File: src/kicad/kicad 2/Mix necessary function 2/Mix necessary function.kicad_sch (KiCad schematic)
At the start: 26 parts, among them SW1 02-JST, SW2 02-JST

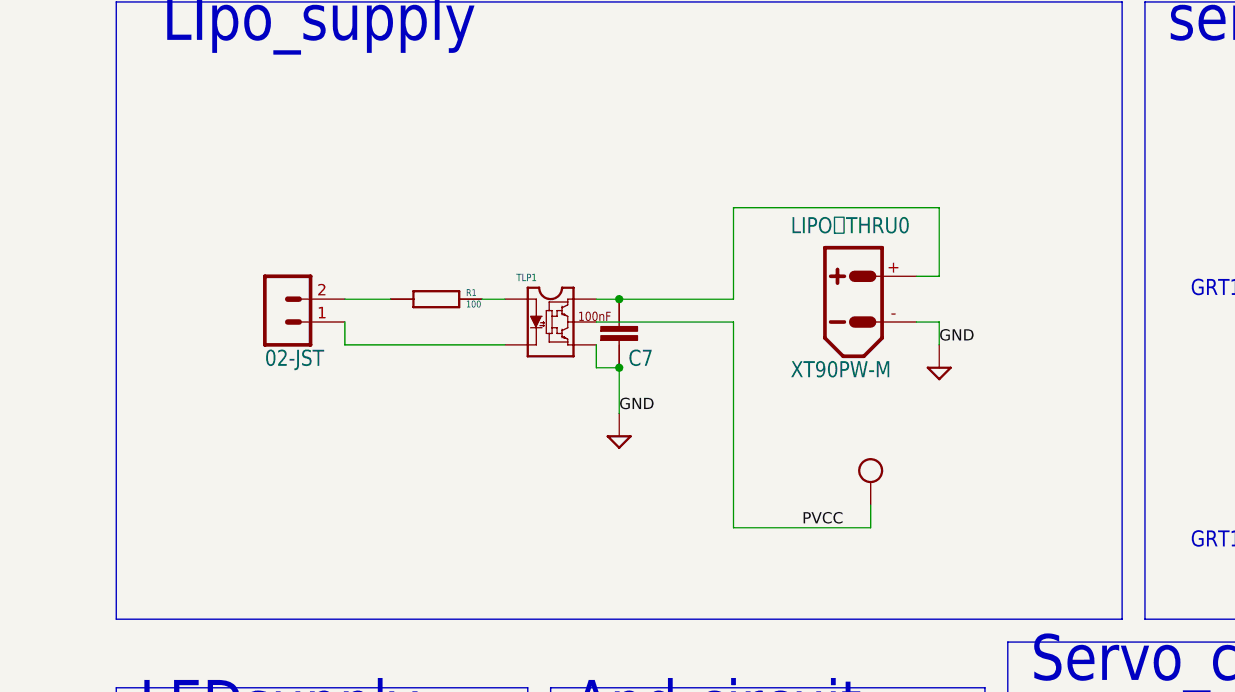
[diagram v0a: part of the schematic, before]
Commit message: fix
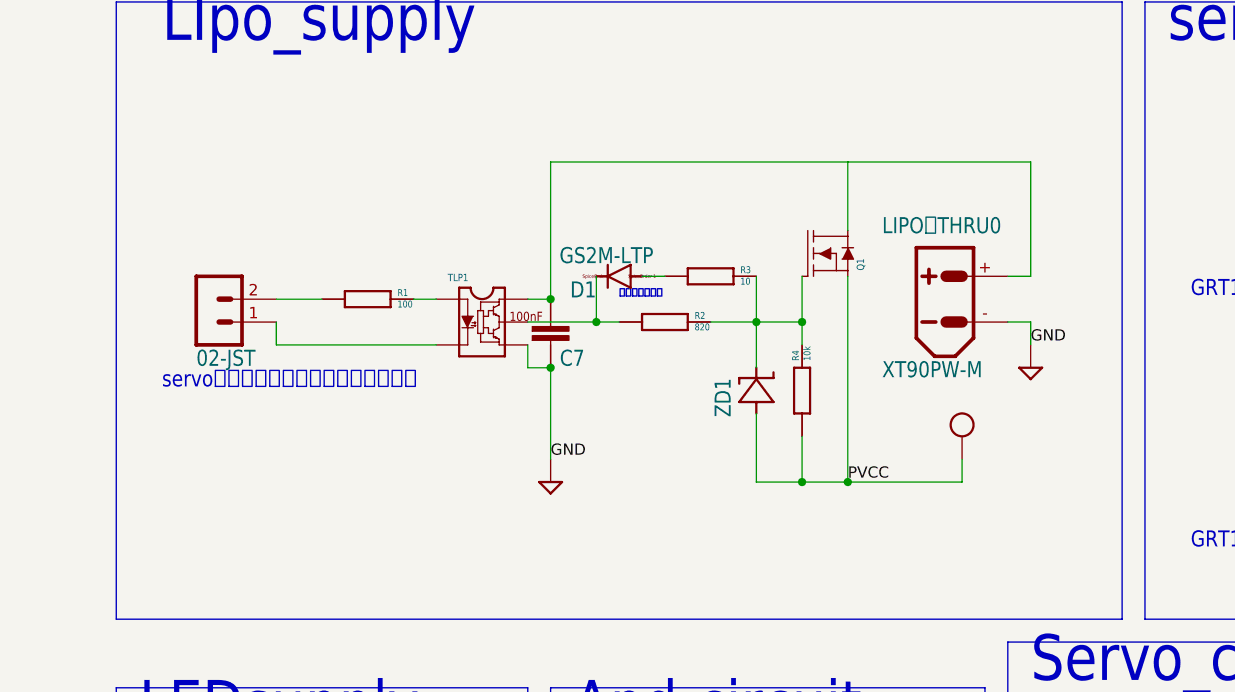
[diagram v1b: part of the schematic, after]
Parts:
- added D1: GS2M-LTP, Mix necessary function:GS2M-LTP, symbol Mix necessary function-eagle-import:GS2M-LTP
- added Q1: SQJA16EP-T1_GE3, Mix necessary function:SQJA16EP-T1_GE3, symbol Mix necessary function-eagle-import:SQJA16EP-T1_GE3
- added R2: 820, Mix necessary function:CR0603, symbol Mix necessary function-eagle-import:CR0603
- added R3: 10, Mix necessary function:CR0603, symbol Mix necessary function-eagle-import:CR0603
- added R4: 10k, Mix necessary function:CR0603, symbol Mix necessary function-eagle-import:CR0603
- added ZD1: MMBZ5248B-TP, Mix necessary function:MMBZ5248B-TP, symbol Mix necessary function-eagle-import:MMBZ5248B-TP
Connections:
- net VCC: now also Q1.S1 (S), Q1.S2 (S), Q1.S3 (S), R4.LEFT, ZD1.ANODE (A); no longer TLP1.VO (VOUT)
- net at C7.P$1, LIPO＿THRU0.+, TLP1.VCC: now also Q1.D
- new net: D1.A, R3.LEFT
- new net: D1.C, R2.LEFT, TLP1.VO (VOUT)
- new net: Q1.G, R2.RIGHT, R3.RIGHT, R4.RIGHT, ZD1.CATHODE (C)
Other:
- note added: "servoの非常停止機能の接続用コネクタ"
- note added: "逆方向漏れ防止"
